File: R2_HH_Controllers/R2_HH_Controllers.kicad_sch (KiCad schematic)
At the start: 27 parts, among them IC1 E22-900M22S, J1 U.FL-R-SMT-1_10_, J2 USB4105-GF-A, J3 S2B-PH-SM4-TB_LF__SN_, SW1 SW_Push, SW10 SW_Push, SW11 SW_Push, SW2 Reset, SW3 Boot, SW4 SW_Push, SW5 PCM12SMTR, SW6 SW_Push, SW7 SW_Push, SW8 SW_Push, SW9 SW_Push, U1 ESP32-S3-WROOM-1, U2 USBLC6-2SC6, U3 BQ24074RGT

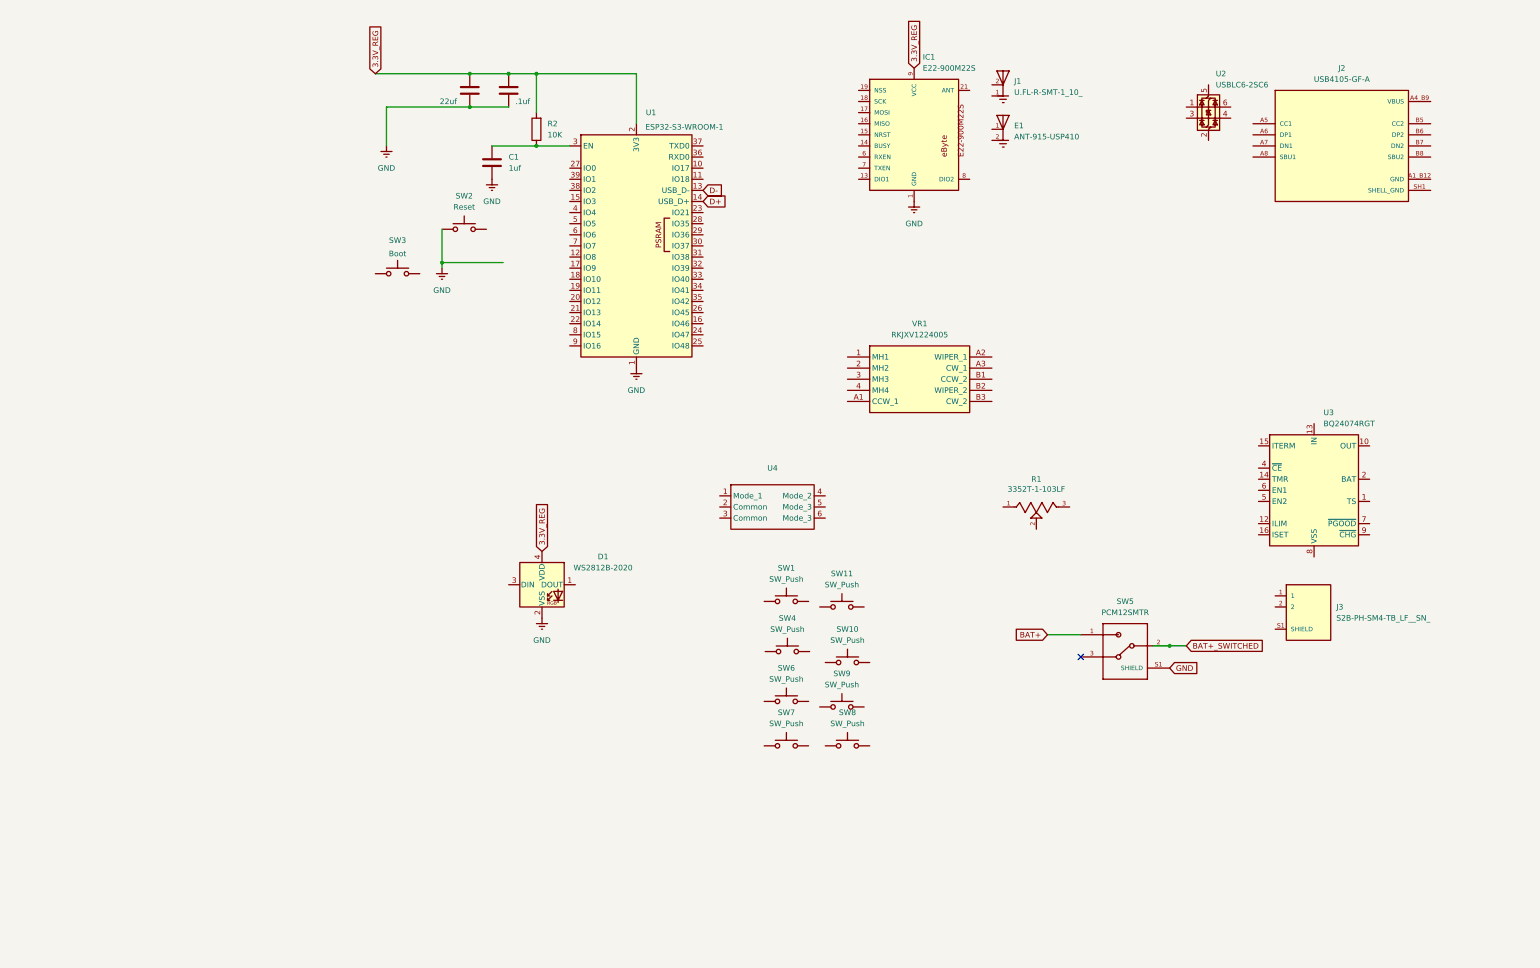
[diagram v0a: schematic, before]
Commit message: hh
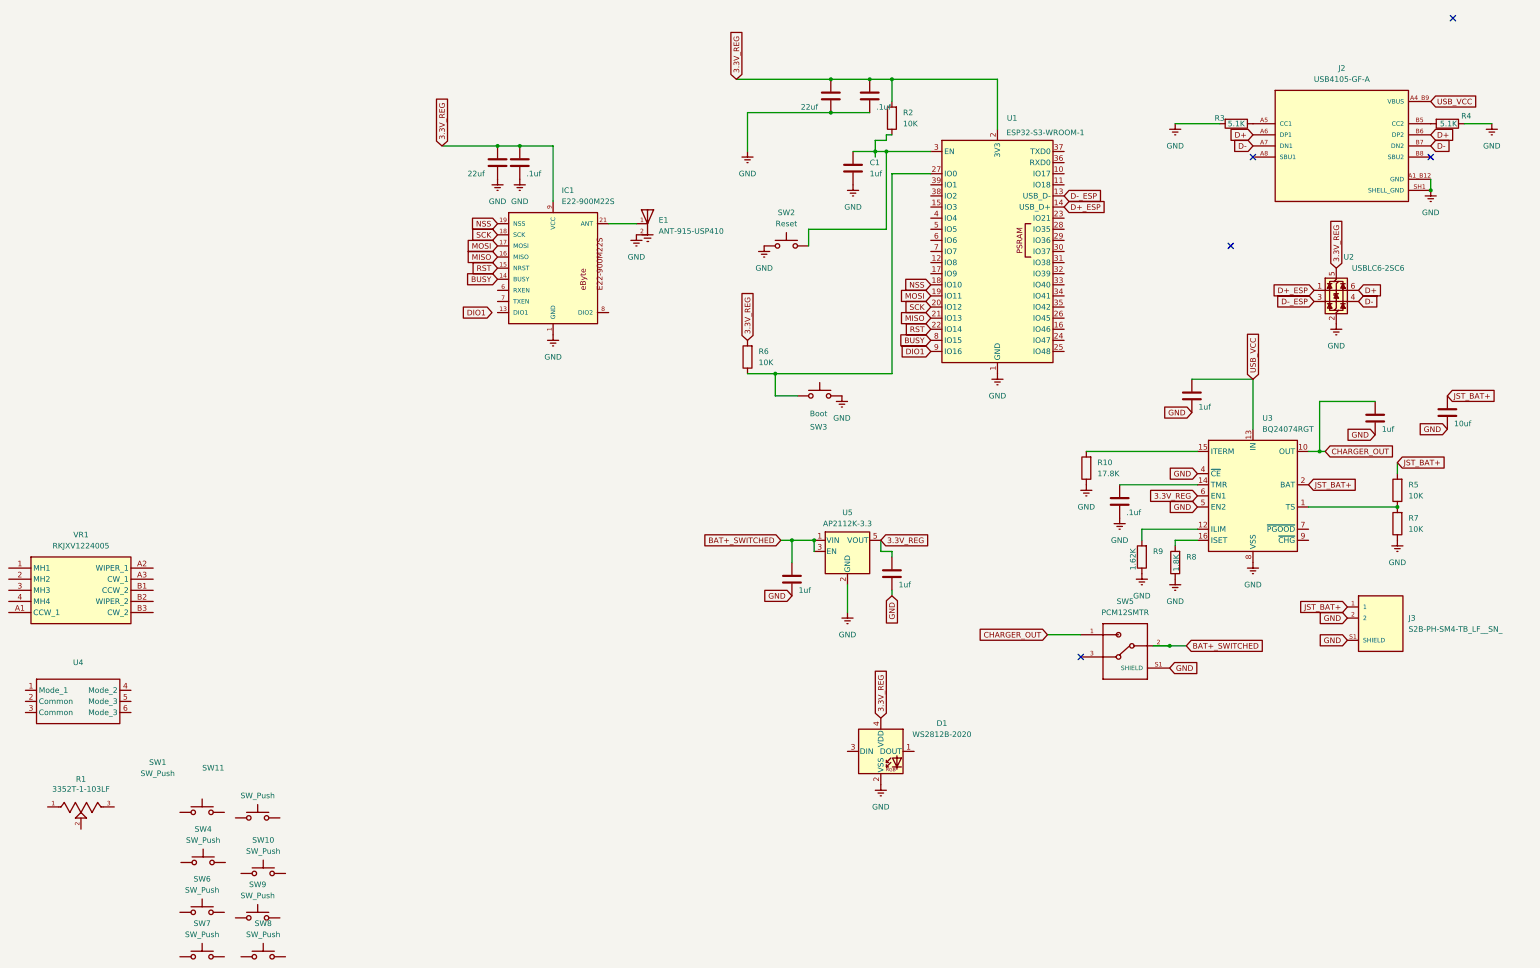
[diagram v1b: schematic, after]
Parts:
- removed J1: U.FL-R-SMT-1_10_, custom:HRS_U.FL-R-SMT-1_10_, symbol 01-Custom:U.FL-R-SMT-1_10_
- added C10: 22uf, Capacitor_SMD:C_0201_0603Metric, symbol Device:C
- added C11, C4: .1uf, Capacitor_SMD:C_0201_0603Metric, symbol Device:C
- added C5, C7, C8, C9: 1uf, Capacitor_SMD:C_0201_0603Metric, symbol Device:C
- added C6: 10uf, Capacitor_SMD:C_0201_0603Metric, symbol Device:C
- added R10: 17.8K, Resistor_SMD:R_0201_0603Metric, symbol Device:R
- added R3, R4: 5.1K, Resistor_SMD:R_0201_0603Metric, symbol Device:R
- added R5, R6, R7: 10K, Resistor_SMD:R_0201_0603Metric, symbol Device:R
- added R8: 1.8K, Resistor_SMD:R_0201_0603Metric, symbol Device:R
- added R9: 1.62K, Resistor_SMD:R_0201_0603Metric, symbol Device:R
- added U5: AP2112K-3.3, Package_TO_SOT_SMD:SOT-23-5, symbol Regulator_Linear:AP2112K-3.3
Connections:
- net BAT+ is gone; now on net CHARGER_OUT: SW5.1
- net SHELL_GND is gone; now on net GND: J2.SH1 (SHELL_GND), J2.SH2 (SHELL_GND), J2.SH3 (SHELL_GND), J2.SH4 (SHELL_GND)
- net 3.3V_REG: now also U2.5 (VBUS), U3.6 (EN1), C10.2, C11.2, C9.2, R6.2, U5.5 (VOUT)
- net BAT+_SWITCHED: now also C8.2, U5.1 (VIN), U5.3 (EN)
- net D+: now also J2.A6 (DP1), J2.B6 (DP2), U2.6 (I/O1); no longer U1.14 (USB_D+)
- net D-: now also J2.A7 (DN1), J2.B7 (DN2), U2.4 (I/O2); no longer U1.13 (USB_D-)
- net GND: now also E1.2, J3.2, J3.S1 (SHIELD), J3.S2 (SHIELD), SW3.2, U2.2 (GND), U3.17 (VSS), U3.4 (~{CE}), U3.5 (EN2), U3.8 (VSS), C10.1, C11.1, C4.1, C5.1, C6.1, C7.1, C8.1, C9.1, R10.1, R3.2, R4.1, R7.1, R8.1, R9.1, U5.2 (GND)
- net VBUS: now also U3.13 (IN), C5.2
- net at U3.1 (TS): now also R5.1, R7.2
- net CHARGER_OUT: now reaches U3.10 (OUT), U3.11 (OUT)
- net CHARGER_OUT: now also C7.2
- net at U3.12 (ILIM): now also R9.2
- net at U3.14 (TMR): now also C4.2
- net at U3.15 (ITERM): now also R10.2
- net at U3.16 (ISET): now also R8.2
- net JST_BAT+: now reaches U3.2 (BAT), U3.3 (BAT)
- net JST_BAT+: now also J3.1, C6.2, R5.2
- net at C1.1, R2.1, U1.3 (EN): now also SW2.2
- net at J2.A5 (CC1): now also R3.1
- net at J2.B5 (CC2): now also R4.2
- net BUSY: now reaches IC1.14 (BUSY)
- net BUSY: now also U1.8 (IO15)
- net RST: now reaches IC1.15 (NRST)
- net RST: now also U1.22 (IO14)
- net MISO: now reaches IC1.16 (MISO)
- net MISO: now also U1.21 (IO13)
- net MOSI: now reaches IC1.17 (MOSI)
- net MOSI: now also U1.19 (IO11)
- net SCK: now reaches IC1.18 (SCK)
- net SCK: now also U1.20 (IO12)
- net NSS: now reaches IC1.19 (NSS)
- net NSS: now also U1.18 (IO10)
- net at IC1.21 (ANT): now also E1.1
- net at SW3.1: now also U1.27 (IO0), R6.1
- net D+_ESP: now reaches U2.1 (I/O1)
- net D+_ESP: now also U1.14 (USB_D+)
- net D-_ESP: now reaches U2.3 (I/O2)
- net D-_ESP: now also U1.13 (USB_D-)
- net DIO1: now reaches U1.9 (IO16)
- no-connect marks 1 -> 5
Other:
- moved on the sheet: C1, D1, E1, IC1, J3, R1, R2, SW1, SW10, SW11, SW2, SW3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
